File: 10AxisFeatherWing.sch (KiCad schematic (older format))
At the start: 23 parts, among them J1 feather long, J2 feather short, J3 feather long, J4 feather short, J5 INT, J6 NRESET, U1 BNO055, U2 BME280, Y1 32.768kHz

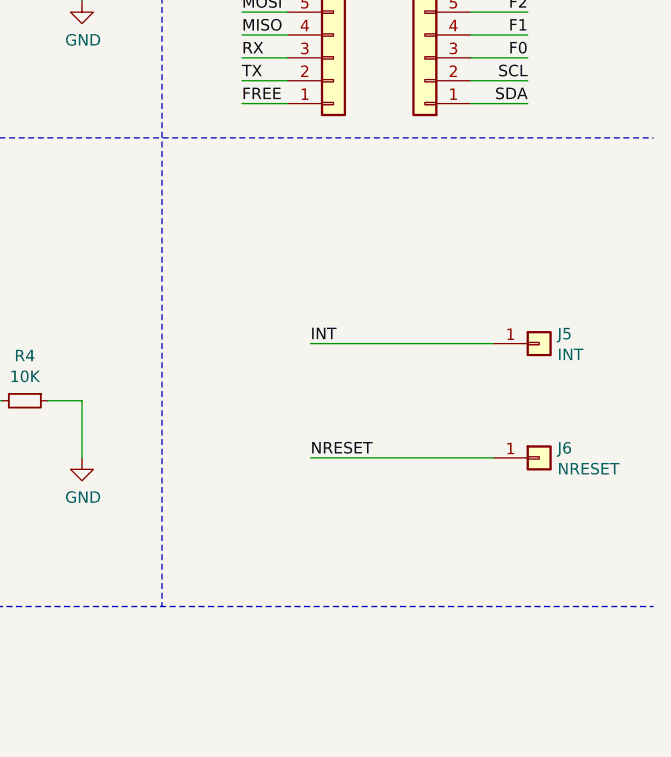
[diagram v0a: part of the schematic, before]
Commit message: Minor format fix
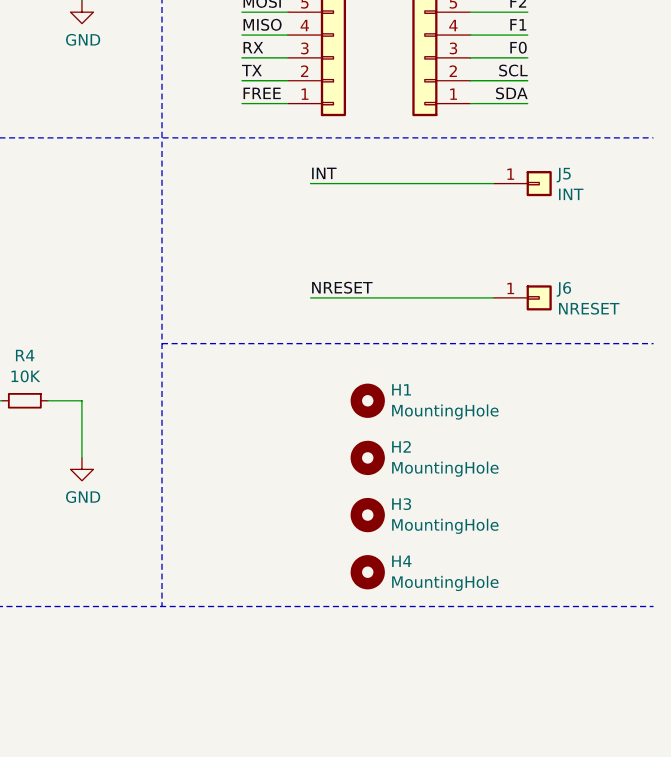
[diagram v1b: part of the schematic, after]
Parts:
- added H1, H2, H3, H4: MountingHole, MountingHole:MountingHole_2.7mm_M2.5, symbol Mechanical:MountingHole
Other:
- moved on the sheet: J5, J6
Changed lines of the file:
@@
 L Connector_Generic:Conn_01x01 J5
 U 1 1 5E233B4E
-P 10000 5500
-F 0 "J5" H 10080 5542 50  0000 L CNN
-F 1 "INT" H 10080 5451 50  0000 L CNN
-F 2 "Connector_Wire:SolderWirePad_1x01_Drill0.8mm" H 10000 5500 50  0001 C CNN
-F 3 "~" H 10000 5500 50  0001 C CNN
-	1    10000 5500
+P 10000 4800
+F 0 "J5" H 10080 4842 50  0000 L CNN
+F 1 "INT" H 10080 4751 50  0000 L CNN
+F 2 "Connector_Wire:SolderWirePad_1x01_Drill0.8mm" H 10000 4800 50  0001 C CNN
+F 3 "~" H 10000 4800 50  0001 C CNN
+	1    10000 4800
 	1    0    0    -1
 $EndComp
-Text Label 9000 5500 0    50   ~ 0
+Text Label 9000 4800 0    50   ~ 0
 INT
 Wire Wire Line
@@
 Wire Notes Line
 	6200 500  6200 8000
-Text Label 9000 6000 0    50   ~ 0
+Text Label 9000 5300 0    50   ~ 0
 NRESET
 $Comp
 L Connector_Generic:Conn_01x01 J6
 U 1 1 5E15A9A2
-P 10000 6000
-F 0 "J6" H 10080 6042 50  0000 L CNN
-F 1 "NRESET" H 10080 5951 50  0000 L CNN
-F 2 "Connector_Wire:SolderWirePad_1x01_Drill0.8mm" H 10000 6000 50  0001 C CNN
-F 3 "~" H 10000 6000 50  0001 C CNN
-	1    10000 6000
+P 10000 5300
+F 0 "J6" H 10080 5342 50  0000 L CNN
+F 1 "NRESET" H 10080 5251 50  0000 L CNN
+F 2 "Connector_Wire:SolderWirePad_1x01_Drill0.8mm" H 10000 5300 50  0001 C CNN
+F 3 "~" H 10000 5300 50  0001 C CNN
+	1    10000 5300
 	1    0    0    -1
 $EndComp
 Wire Wire Line
-	9000 5500 9800 5500
+	9000 4800 9800 4800
 Wire Wire Line
-	9000 6000 9800 6000
+	9000 5300 9800 5300
 Wire Wire Line
 	6500 2000 7750 2000
@@
 Wire Wire Line
 	7250 1500 7250 1350
+$Comp
+L Mechanical:MountingHole H1
+U 1 1 5E165FBB
+P 9250 5750
+F 0 "H1" H 9350 5796 50  0000 L CNN
+F 1 "MountingHole" H 9350 5705 50  0000 L CNN
+F 2 "MountingHole:MountingHole_2.7mm_M2.5" H 9250 5750 50  0001 C CNN
+F 3 "~" H 9250 5750 50  0001 C CNN
+	1    9250 5750
+	1    0    0    -1
+$EndComp
+$Comp
+L Mechanical:MountingHole H2
+U 1 1 5E16676B
+P 9250 6000
+F 0 "H2" H 9350 6046 50  0000 L CNN
+F 1 "MountingHole" H 9350 5955 50  0000 L CNN
+F 2 "MountingHole:MountingHole_2.7mm_M2.5" H 9250 6000 50  0001 C CNN
+F 3 "~" H 9250 6000 50  0001 C CNN
+	1    9250 6000
+	1    0    0    -1
+$EndComp
+$Comp
+L Mechanical:MountingHole H3
+U 1 1 5E166D96
+P 9250 6250
+F 0 "H3" H 9350 6296 50  0000 L CNN
+F 1 "MountingHole" H 9350 6205 50  0000 L CNN
+F 2 "MountingHole:MountingHole_2.7mm_M2.5" H 9250 6250 50  0001 C CNN
+F 3 "~" H 9250 6250 50  0001 C CNN
+	1    9250 6250
+	1    0    0    -1
+$EndComp
+$Comp
+L Mechanical:MountingHole H4
+U 1 1 5E16742A
+P 9250 6500
+F 0 "H4" H 9350 6546 50  0000 L CNN
+F 1 "MountingHole" H 9350 6455 50  0000 L CNN
+F 2 "MountingHole:MountingHole_2.7mm_M2.5" H 9250 6500 50  0001 C CNN
+F 3 "~" H 9250 6500 50  0001 C CNN
+	1    9250 6500
+	1    0    0    -1
+$EndComp
+Wire Notes Line
+	8350 5500 10500 5500
 $EndSCHEMATC
